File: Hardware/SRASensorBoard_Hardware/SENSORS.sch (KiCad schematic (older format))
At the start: 23 parts

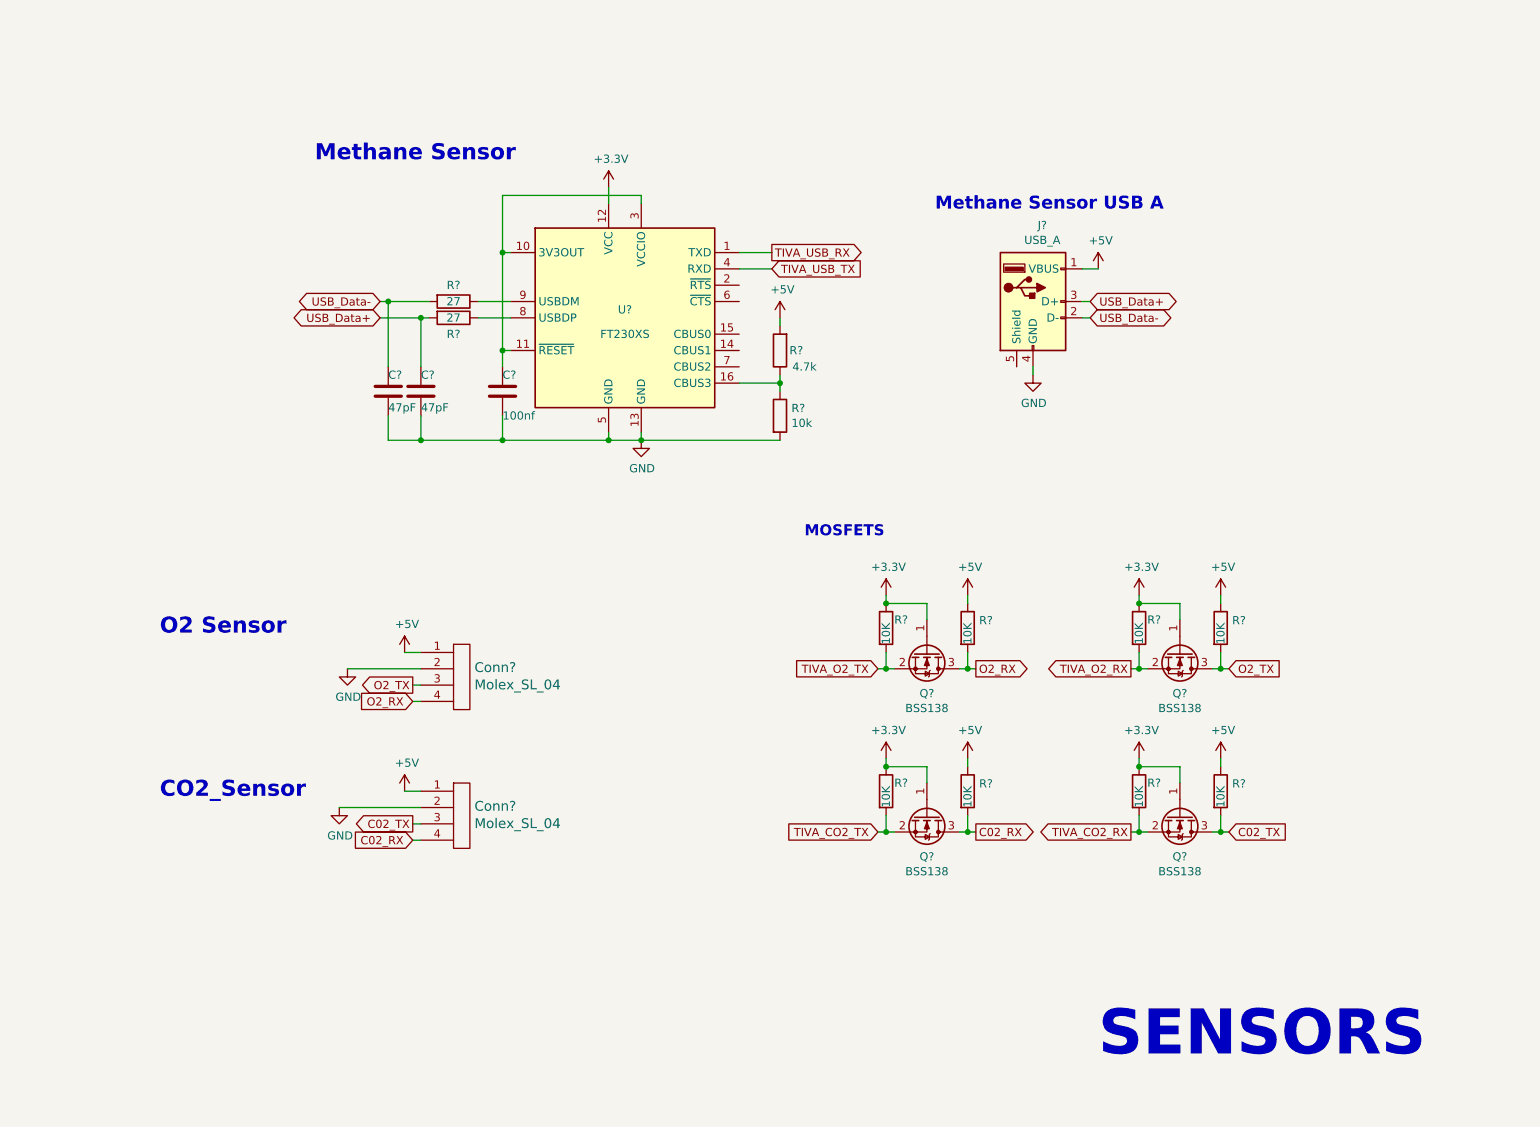
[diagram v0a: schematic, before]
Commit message: Sciency stuff for the board
finished!
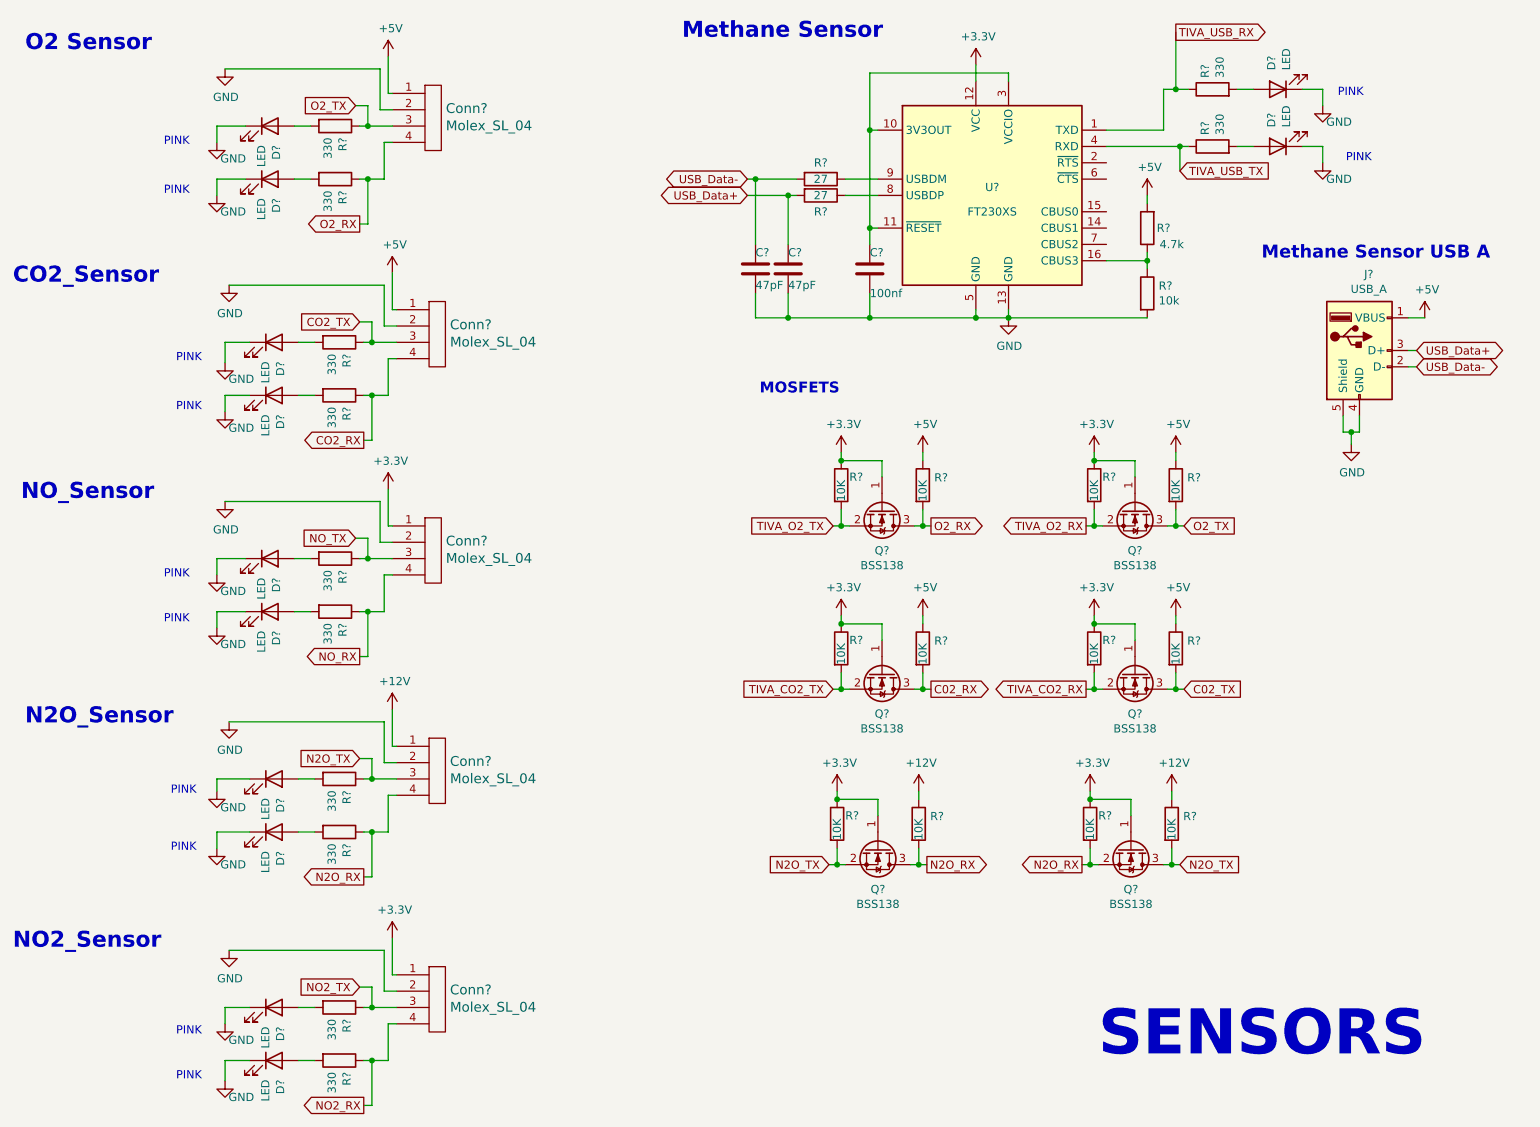
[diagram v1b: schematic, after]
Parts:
- removed Conn?: Molex_SL_04, MRDT_Connectors:MOLEX_SL_04_Vertical, symbol MRDT_Connectors:Molex_SL_04
- added Conn? (x4): Molex_SL_04, MRDT_Connectors:MOLEX_SL_04_Vertical, symbol MRDT_Connectors:Molex_SL_04
- added D? (x12): LED, Diode_SMD:D_0603_1608Metric_Pad1.05x0.95mm_HandSolder, symbol Device:LED
- added Q? (x2): BSS138, Package_TO_SOT_SMD:SOT-23, symbol Transistor_FET:BSS138
- added R? (x4): 10K, Resistor_SMD:R_0603_1608Metric_Pad1.05x0.95mm_HandSolder, symbol Device:R
- added R? (x12): 330, Resistor_SMD:R_0603_1608Metric_Pad1.05x0.95mm_HandSolder, symbol Device:R
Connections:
- net +3V3: now also Conn?.1, Conn?.1, Q?.1 (G), Q?.1 (G), R?.1, R?.1
- net +5V: now also Conn?.1
- net GND: now also J?.5 (Shield), Conn?.2, Conn?.2, Conn?.2, Conn?.2, D?.1 (K), D?.1 (K), D?.1 (K), D?.1 (K), D?.1 (K), D?.1 (K), D?.1 (K), D?.1 (K), D?.1 (K), D?.1 (K), D?.1 (K), D?.1 (K)
- net O2_RX: now also R?.1
- net O2_TX: now also R?.1
- net TIVA_USB_RX: now also R?.1
- net TIVA_USB_TX: now also R?.1
- new net: D?.2 (A), R?.2 (x12)
- new net +12V: Conn?.1, R?.1, R?.1
- new net CO2_RX: Conn?.4, R?.1
- new net CO2_TX: Conn?.3, R?.1
- new net N2O_RX: Conn?.4, Q?.2 (S), Q?.3 (D), R?.1, R?.2, R?.2
- new net N2O_TX: Conn?.3, Q?.2 (S), Q?.3 (D), R?.1, R?.2, R?.2
- new net NO2_RX: Conn?.4, R?.1
- new net NO2_TX: Conn?.3, R?.1
- new net NO_RX: Conn?.4, R?.1
- new net NO_TX: Conn?.3, R?.1
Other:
- note added: "N2O_Sensor\n"
- note added: "NO2_Sensor\n"
- note added: "NO_Sensor"
- note added: "PINK"
- note added: "PINK\n"
- moved on the sheet: C?, Conn?, J?, Q?, R?, U?
